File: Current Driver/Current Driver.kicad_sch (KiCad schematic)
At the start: 41 parts, among them Q1 BC817, Q2 D45H11G (n_b), Q3 BC807, Q4 D44H11(n_b), SW1 SW_Push, U1 ADA4622-2xCP, U2 ADA4622-2xCP

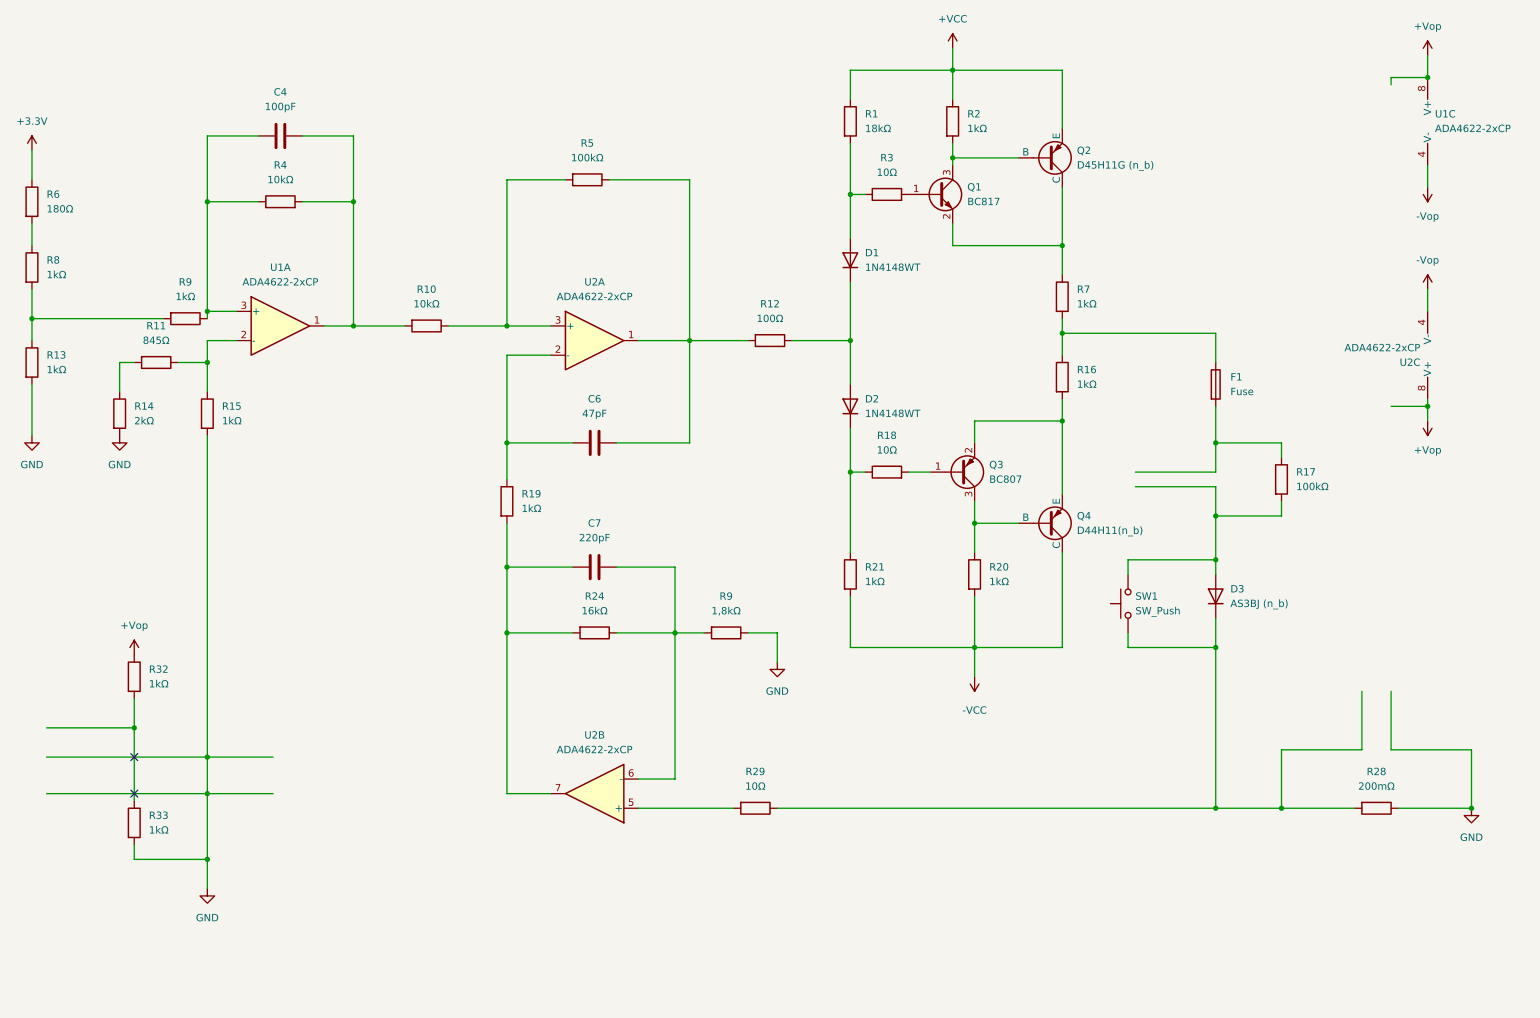
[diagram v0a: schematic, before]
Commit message: Clean Schematic
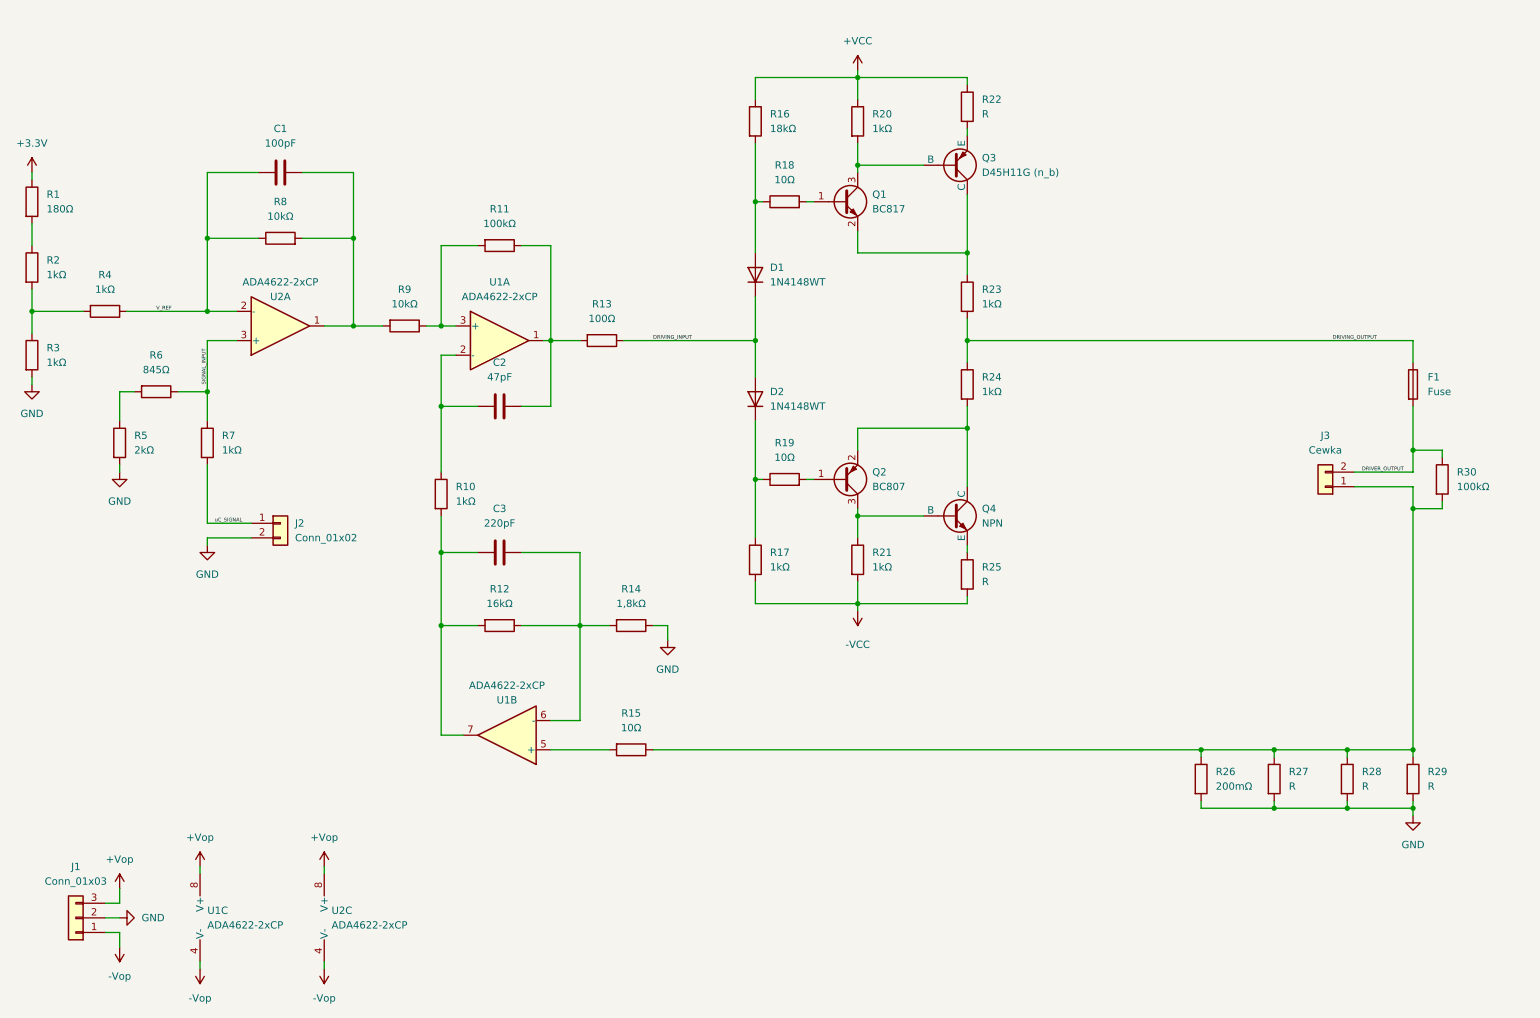
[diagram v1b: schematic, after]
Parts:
- removed D3: AS3BJ (n_b), Diode_SMD:D_SOD-523, symbol Diode:1N4148WT
- removed Q4: D44H11(n_b), symbol Simulation_SPICE:PNP
- removed R32, R33: 1kΩ, symbol Device:R
- removed SW1: SW_Push, symbol Switch:SW_Push
- removed unit 2 of U2
- added J1: Conn_01x03, symbol Connector_Generic:Conn_01x03
- added J2: Conn_01x02, symbol Connector_Generic:Conn_01x02
- added J3: Cewka, symbol Connector_Generic:Conn_01x02
- added Q4: NPN, symbol Simulation_SPICE:NPN
- added R22, R25, R27, R28, R29: R, symbol Device:R
- added unit 2 of U1
- renumbered C4 to C1, C6 to C2, C7 to C3, Q3 to Q2, Q2 to Q3, R6 to R1, R19 to R10, R5 to R11, R24 to R12, R12 to R13, R9 to R14, R29 to R15, R1 to R16, R21 to R17, R3 to R18, R18 to R19, R8 to R2, R2 to R20, R20 to R21, R7 to R23, R16 to R24, R28 to R26, R13 to R3, R17 to R30, R9 to R4, R14 to R5, R11 to R6, R15 to R7, R4 to R8, R10 to R9
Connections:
- net +VCC: now also R22.1; no longer Q3.3 (E)
- net +Vop: now also J1.3 (Pin_3)
- net -VCC: now also R25.2
- net -Vop: now also J1.1 (Pin_1)
- net GND: now also R26.2, J1.2 (Pin_2), J2.2 (Pin_2), R27.2, R28.2, R29.2; no longer R26.1, R7.2
- net DRIVING_OUTPUT: now reaches F1.1, R23.2, R24.1
- net DRIVER_OUTPUT: now reaches F1.2, R30.1
- net DRIVER_OUTPUT: now also J3.2 (Pin_2)
- net at Q2.2 (E), R24.2: now also Q4.1 (C)
- net at Q2.3 (C), R21.1: now also Q4.2 (B)
- net at R30.2: now also R15.1, R26.1, J3.1 (Pin_1), R27.1, R28.1, R29.1
- net at C1.2, R8.2, R9.2: now also U2.1; no longer U1.1
- net SIGNAL_INPUT: now reaches R6.1, R7.1
- net SIGNAL_INPUT: now also U2.3 (+); no longer U1.2 (-)
- net V_REF: now reaches C1.1, R4.1, R8.1
- net V_REF: now also U2.2 (-); no longer U1.3 (+)
- net at C2.1, R10.1: now also U1.2 (-); no longer U2.2 (-)
- net at C2.2, R11.1, R13.2: now also U1.1; no longer U2.1
- net at R11.2, R9.1: now also U1.3 (+); no longer U2.3 (+)
- net at C3.1, R10.2, R12.2: now also U1.7
- net at C3.2, R12.1, R14.2: now also U1.6 (-)
- net DRIVING_INPUT: now reaches D1.1 (K), D2.2 (A), R13.1
- net at R15.2: now also U1.5 (+)
- new net: Q3.3 (E), R22.2
- new net: Q4.3 (E), R25.1
- new net uC_SIGNAL: J2.1 (Pin_1), R7.2
- no-connect marks 2 -> 0
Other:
- company: (none) -> KN NaMi
- moved on the sheet: C1, C2, C3, D1, D2, F1, Q1, Q2, Q3, R10, R11, R12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
